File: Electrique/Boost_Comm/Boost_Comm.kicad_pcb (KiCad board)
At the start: 2 copper layers, 21 parts, among them M1 CSD17571Q2, U1 TPS40210DGQ

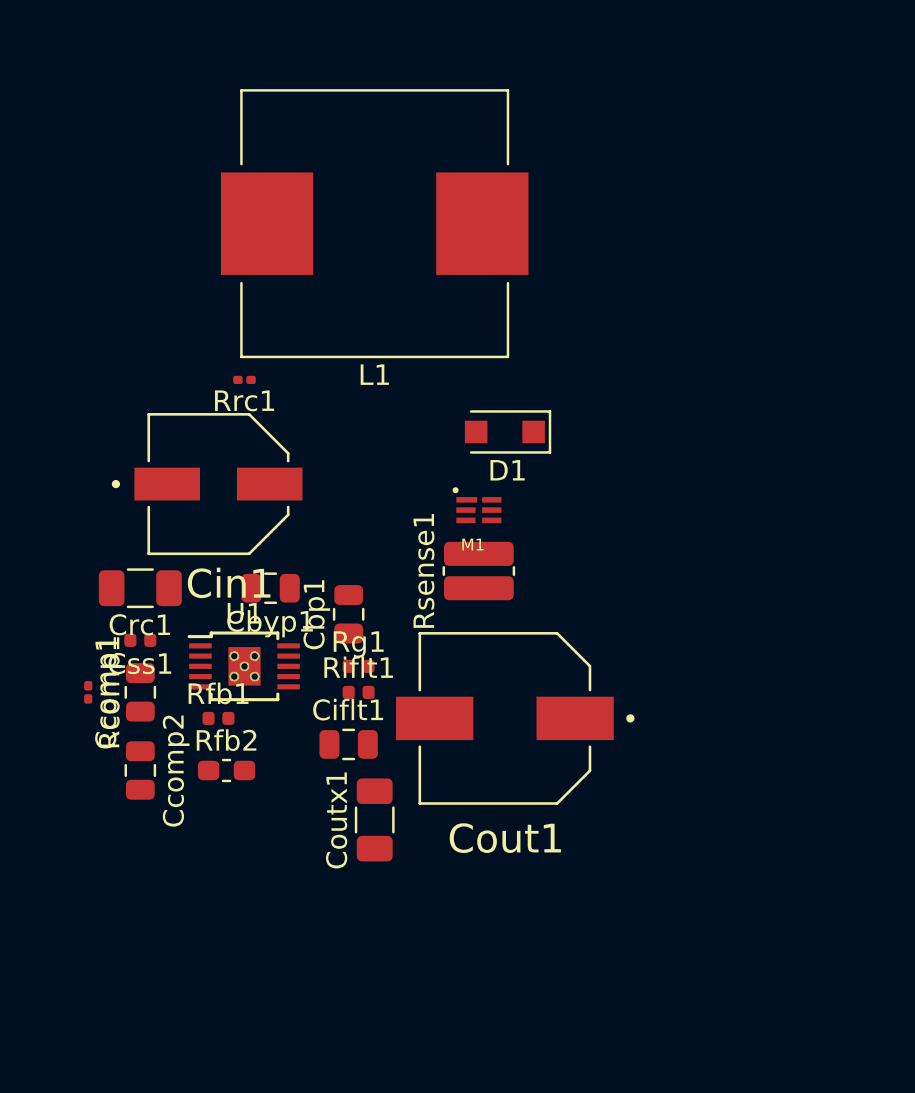
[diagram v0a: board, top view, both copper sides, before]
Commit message: Pcb trace boost update
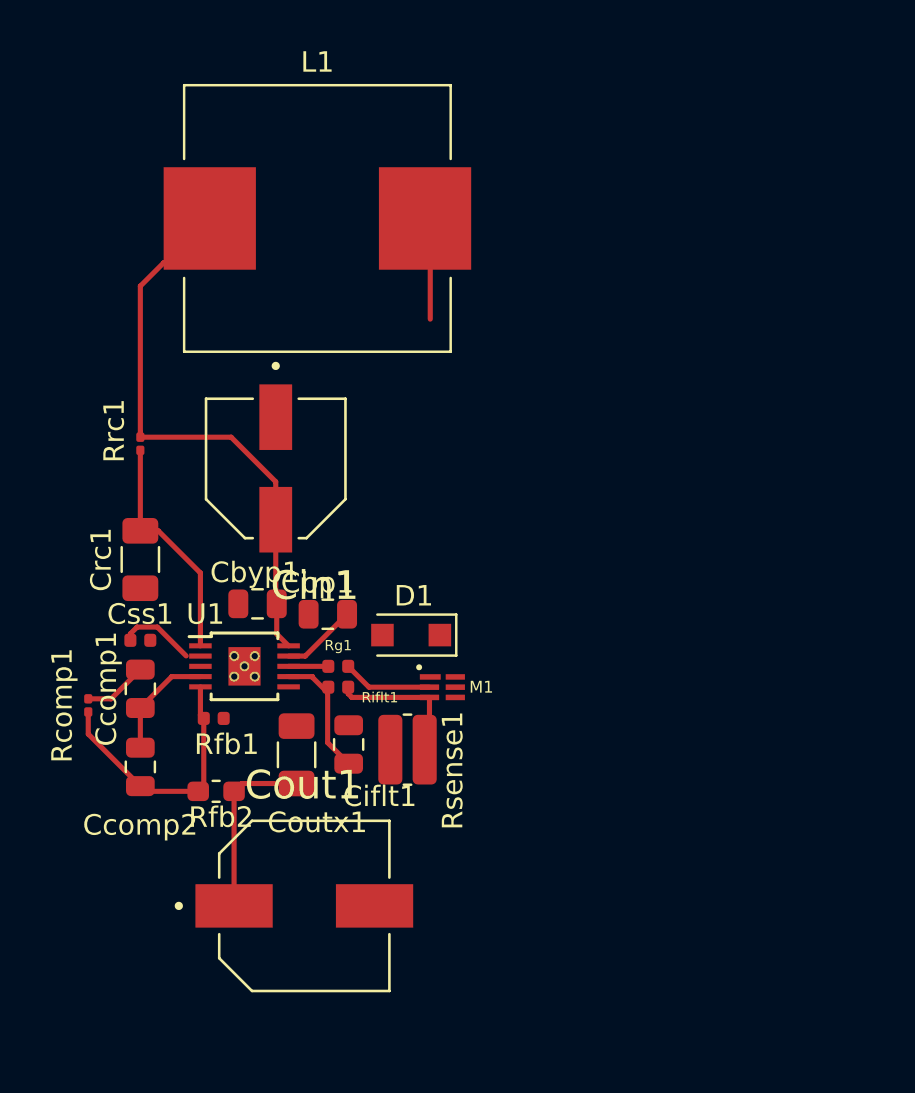
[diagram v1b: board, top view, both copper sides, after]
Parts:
- moved Cout1 13.4 mm to (160.4, 118.4), turned to 0 degrees
- moved D1 10.9 mm to (165.6, 105.2)
- moved Rsense1 9.38 mm to (165.4, 110.7), turned to 0 degrees
- moved M1 8.82 mm to (167.1, 107.7)
- moved Rrc1 5.96 mm to (152.4, 95.8), turned to 270 degrees
- moved Coutx1 4.96 mm to (160.0, 111.0)
- moved Cin1 2.90 mm to (159.0, 97.0), turned to 90 degrees
- moved L1 2.81 mm to (161.0, 84.8)
- moved Crc1 1.40 mm to (152.4, 101.5), turned to 270 degrees
- moved Rfb2 1.14 mm to (156.1, 112.8)
- moved Riflt1 1.02 mm to (162.1, 107.7)
- moved Cbp1 1.02 mm to (161.5, 104.1), turned to 180 degrees
- moved Rg1 0.99 mm to (162.1, 106.7)
- moved Cbyp1 0.99 mm to (158.1, 103.6)
- moved Rcomp1 0.63 mm to (149.9, 108.6)
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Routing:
- net +BATT: track 0.00 -> 27.2 mm
- net Net-(Ccomp2-Pad2): track 0.00 -> 13.2 mm
- net Net-(Crc1-Pad1): track 0.00 -> 11.3 mm
- net Net-(Cout1-Pad1): track 0.00 -> 9.67 mm
- net Net-(M1-Pad3): track 0.00 -> 7.00 mm
- net Net-(Ciflt1-Pad1): track 0.00 -> 6.14 mm
- net Net-(Ccomp1-Pad1): track 0.00 -> 5.50 mm
- net Net-(M1-Pad2): track 0.00 -> 4.39 mm
- net Net-(Css1-Pad1): track 0.00 -> 3.76 mm
- net Net-(Cbp1-Pad1): track 0.00 -> 3.70 mm
- net Net-(Ccomp1-Pad2): track 0.00 -> 3.13 mm
- net Net-(D1-Pad2): track 0.00 -> 2.75 mm
- net Net-(Rg1-Pad1): track 0.00 -> 1.94 mm

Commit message: Update PCB
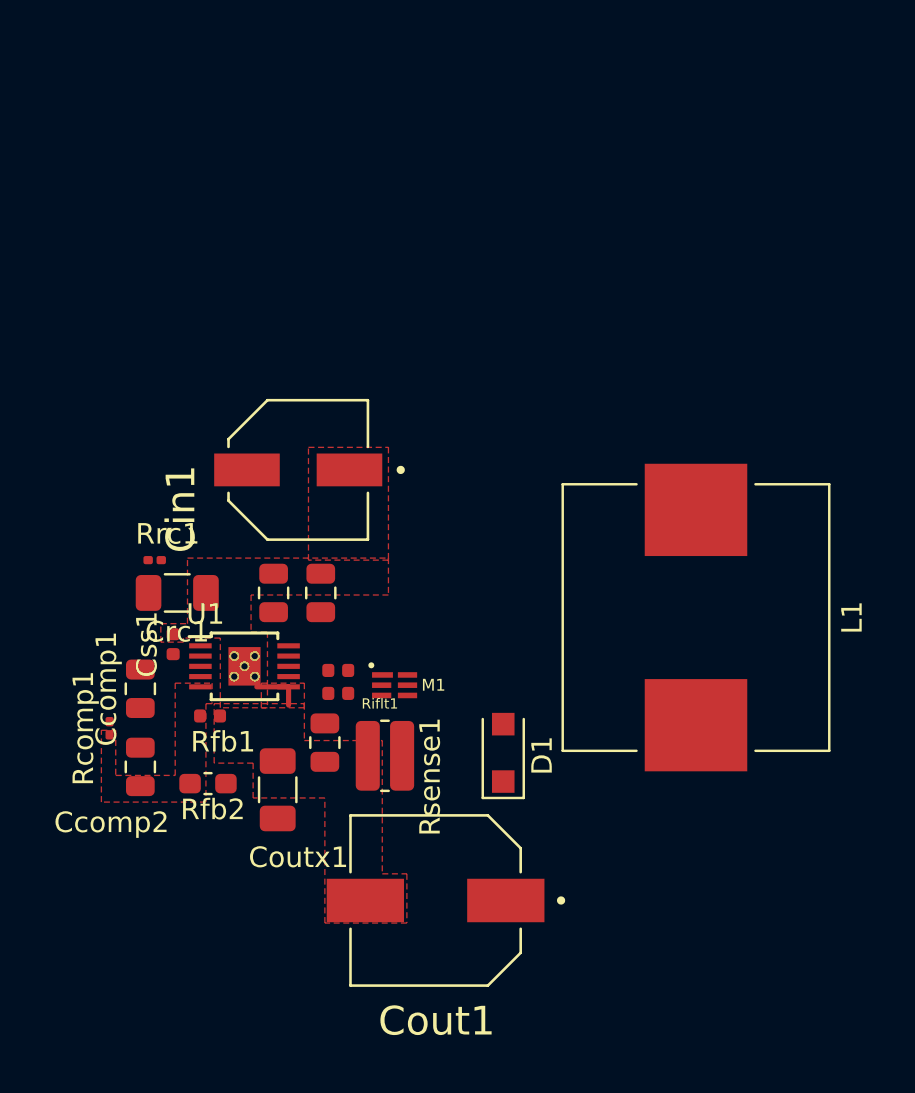
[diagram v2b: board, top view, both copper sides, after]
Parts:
- moved L1 26.8 mm to (179.5, 104.3), turned to 90 degrees
- moved D1 7.29 mm to (170.1, 110.9), turned to 90 degrees
- moved Cout1 6.41 mm to (166.8, 118.1), turned to 180 degrees
- moved Rrc1 5.72 mm to (153.1, 101.5), turned to 180 degrees
- moved Cbyp1 3.13 mm to (161.2, 103.1), turned to 90 degrees
- moved Cbp1 2.84 mm to (158.9, 103.1), turned to 90 degrees
- moved Crc1 2.43 mm to (154.2, 103.1), turned to 0 degrees
- moved M1 2.33 mm to (164.8, 107.6)
- moved Coutx1 1.94 mm to (159.1, 112.7)
- moved Css1 1.61 mm to (154.0, 105.6), turned to 90 degrees
- moved Rcomp1 1.52 mm to (150.9, 109.7)
- moved Ciflt1 1.16 mm to (161.4, 110.4), turned to 270 degrees
- moved Rsense1 1.14 mm to (164.3, 111.0)
- moved Cin1 1.10 mm to (160.1, 97.1), turned to 0 degrees
- moved Rfb2 0.55 mm to (155.7, 112.4)
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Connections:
- M1 pad 4: (no net) -> Net-(M1-Pad3)
- M1 pad 5: (no net) -> Net-(M1-Pad2)
- M1 pad 6: (no net) -> Net-(D1-Pad2)
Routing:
- net +BATT: track 27.2 -> 0.00 mm
- net Net-(Ccomp2-Pad2): track 13.2 -> 0.43 mm
- net Net-(Crc1-Pad1): track 11.3 -> 0.00 mm
- net Net-(Cout1-Pad1): track 9.67 -> 0.00 mm
- net Net-(M1-Pad3): track 7.00 -> 0.33 mm
- net Net-(Ciflt1-Pad1): track 6.14 -> 0.00 mm
- net Net-(Ccomp1-Pad1): track 5.50 -> 0.00 mm
- net Net-(M1-Pad2): track 4.39 -> 0.00 mm
- net Net-(Css1-Pad1): track 3.76 -> 0.00 mm
- net Net-(Cbp1-Pad1): track 3.70 -> 0.00 mm
- net Net-(D1-Pad2): track 2.75 -> 0.00 mm
- net Net-(Ccomp1-Pad2): track 3.13 -> 0.39 mm
- net GND: track 0.00 -> 2.44 mm
- net Net-(Rg1-Pad1): track 1.94 -> 0.00 mm
- added copper zone on F.Cu, net GND
- added copper zone on F.Cu, net Net-(Ccomp2-Pad2)
